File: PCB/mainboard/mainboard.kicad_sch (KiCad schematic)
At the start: 14 parts

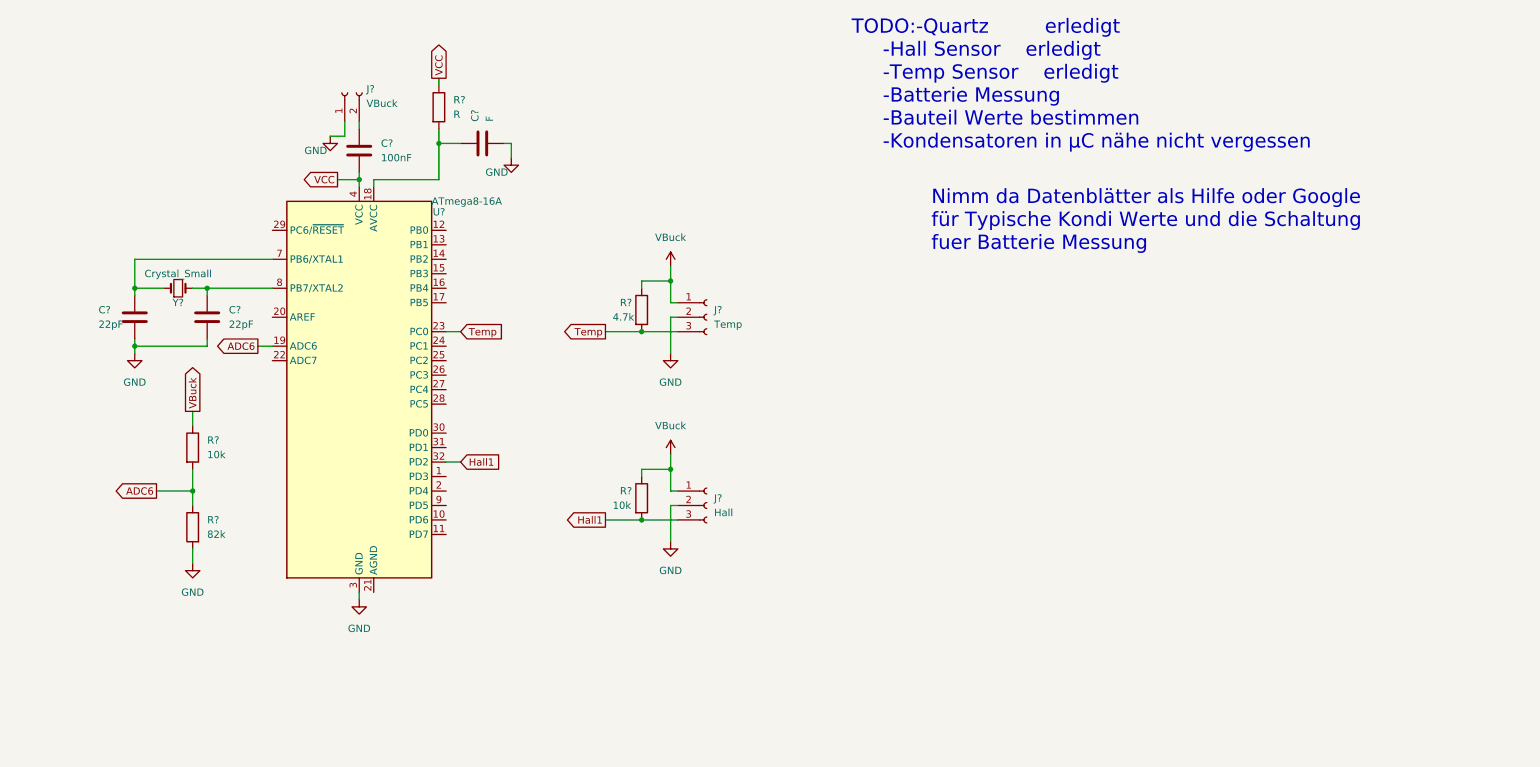
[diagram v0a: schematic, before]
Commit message: Add files via upload
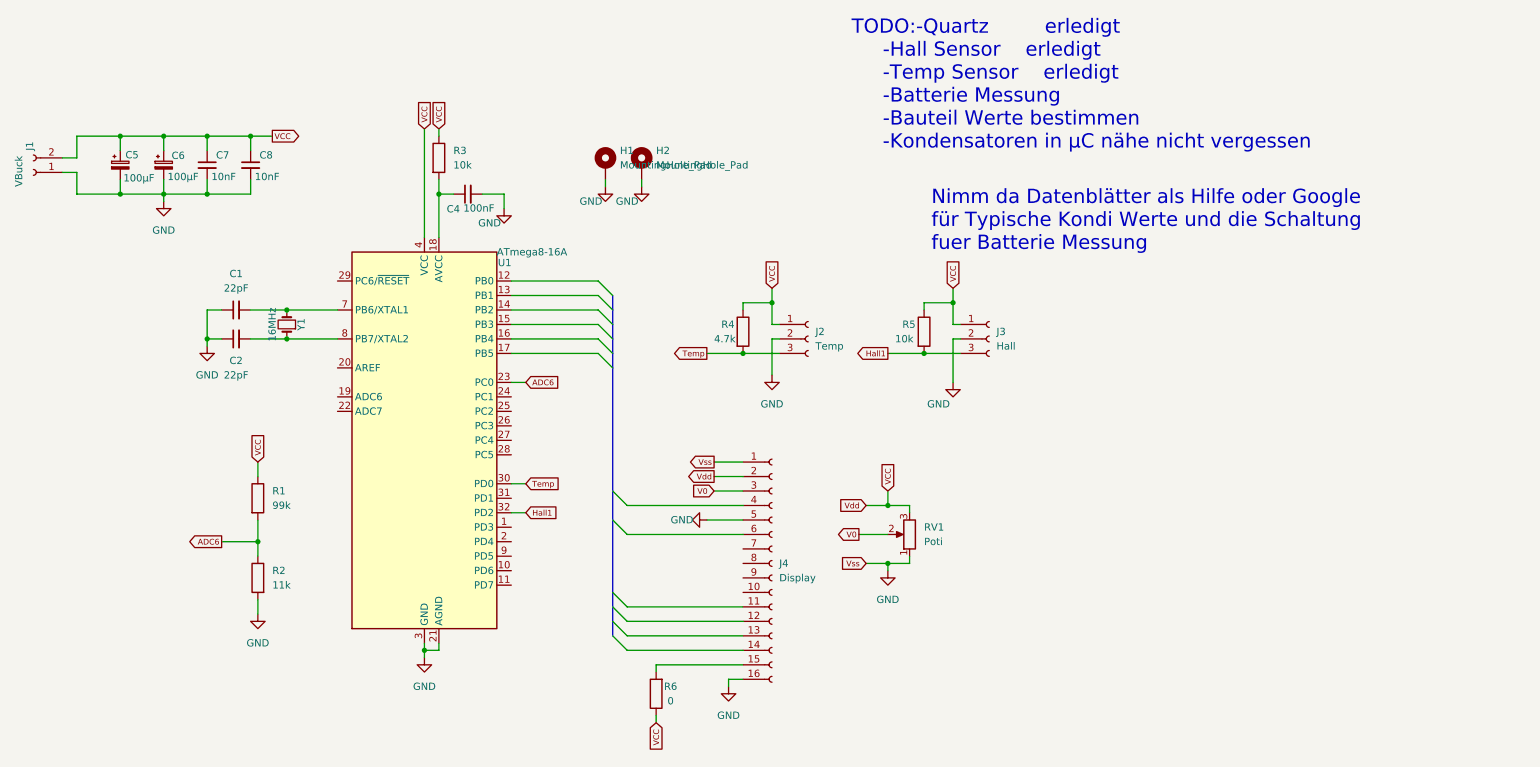
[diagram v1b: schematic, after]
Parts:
- removed C?: F, symbol Device:C
- removed C? (x2): 22pF, symbol Device:C
- removed C?: 100nF, symbol Device:C
- added C1, C2: 22pF, Capacitor_SMD:C_0805_2012Metric, symbol Device:C_Small
- added C4: 100nF, Capacitor_SMD:C_0805_2012Metric, symbol Device:C_Small
- added C5, C6: 100µF, Capacitor_SMD:CP_Elec_5x5.8, symbol Device:C_Polarized_Small
- added C7, C8: 10nF, Capacitor_SMD:C_0603_1608Metric, symbol Device:C_Small
- added H1, H2: MountingHole_Pad, MountingHole:MountingHole_2.7mm_M2.5_Pad, symbol Mechanical:MountingHole_Pad
- added J4: Display, Connector_PinSocket_2.54mm:PinSocket_1x16_P2.54mm_Vertical, symbol Connector:Conn_01x16_Female
- added R6: 0, Resistor_SMD:R_0805_2012Metric, symbol Device:R
- added RV1: Poti, Potentiometer_SMD:Potentiometer_Bourns_3314G_Vertical, symbol Device:R_Potentiometer
- J1: renamed from J?; footprint (none) -> Connector_PinSocket_2.54mm:PinSocket_1x02_P2.54mm_Vertical
- J2, J3: renamed from J?; footprint (none) -> Connector_PinSocket_2.54mm:PinSocket_1x03_P2.54mm_Horizontal
- R1: renamed from R?; value 10k -> 99k; footprint (none) -> Resistor_SMD:R_0805_2012Metric
- R2: renamed from R?; value 82k -> 11k; footprint (none) -> Resistor_SMD:R_0805_2012Metric
- R3: renamed from R?; value R -> 10k; footprint (none) -> Resistor_SMD:R_0805_2012Metric
- R4, R5: renamed from R?; footprint (none) -> Resistor_SMD:R_0805_2012Metric
- Y1: renamed from Y?; value Crystal_Small -> 16MHz; footprint (none) -> Crystal:Crystal_SMD_ECS_CSM3X-2Pin_7.6x4.1mm
- gave numbers to parts that had none: 1
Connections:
- net VBuck is gone; now on net VCC: J2.1 (Pin_1), J3.1 (Pin_1), R1.1, R4.1, R5.1
- net ADC6: now also U1.23 (PC0); no longer U1.19 (ADC6)
- net GND: now also U1.21 (AGND), C1.1, C2.1, C4.2, C5.2, C6.2, C7.2, C8.2, H1.1, H2.1, J4.1 (Pin_1), J4.16 (Pin_16), J4.5 (Pin_5), RV1.1
- net Temp: now also U1.30 (PD0); no longer U1.23 (PC0)
- net VCC: now also J1.2 (Pin_2), C5.1, C6.1, C7.1, C8.1, J4.2 (Pin_2), R6.1, RV1.3
- net at Y1.1: now also U1.8 (PB7/XTAL2), C2.2; no longer U1.7 (PB6/XTAL1)
- net at Y1.2: now also U1.7 (PB6/XTAL1), C1.2; no longer U1.8 (PB7/XTAL2)
- net at R3.2, U1.18 (AVCC): now also C4.1
- new net: J4.15 (Pin_15), R6.2
- new net V0: J4.3 (Pin_3), RV1.2
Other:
- moved on the sheet: J1, J2, J3, R1, R2, R3, R4, R5, U1, Y1
